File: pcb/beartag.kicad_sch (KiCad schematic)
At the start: 25 parts, among them J1 USB_C_Receptacle_USB2.0_14P, Q1 AO3401A, SW1 SW_Push, SW2 SW_Push, U1 CH571F, U2 XC6206P332MR, Y1 32 MHz, Y2 32.768 kHz

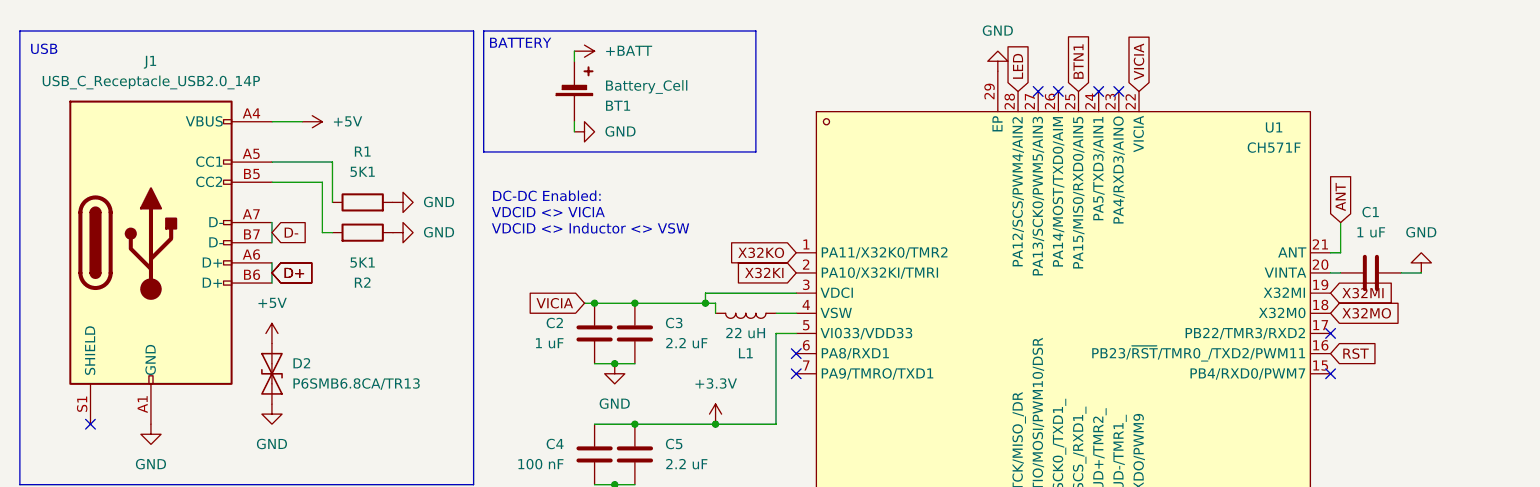
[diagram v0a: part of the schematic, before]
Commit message: pcb updates
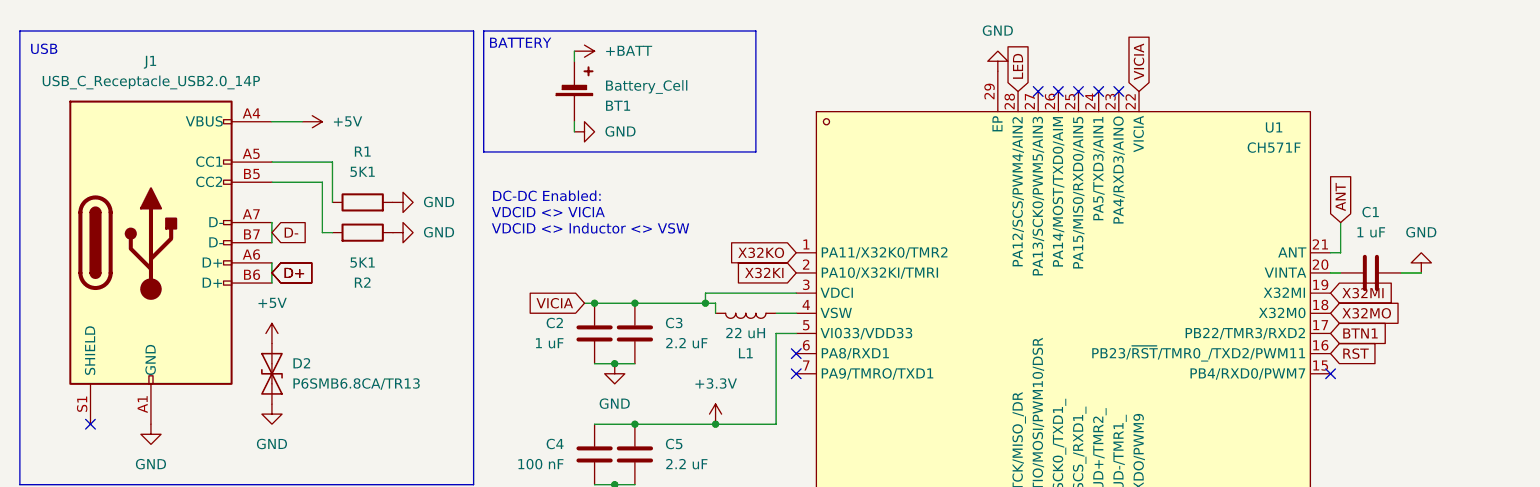
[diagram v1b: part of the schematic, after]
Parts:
- D3: LCSC (none) -> C2286
- R3: LCSC C2286 -> C25905
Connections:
- net BTN1: now also U1.17 (PB22/TMR3/RXD2); no longer U1.25 (PA15/MIS0/RXD0/AIN5)
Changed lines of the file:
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@@
 (kicad_sch
-	(version 20231120)
+	(version 20250114)
 	(generator "eeschema")
-	(generator_version "8.0")
+	(generator_version "9.0")
 	(paper "A4")
+	(rectangle
+		(start 219.71 13.97)
+		(end 252.73 33.02)
+		(stroke
+			(width 0)
+			(type default)
+		)
+		(fill
+			(type none)
+		)
+	)
+	(rectangle
+		(start 100.33 95.25)
+		(end 144.78 128.27)
+		(stroke
+			(width 0)
+			(type default)
+		)
+		(fill
+			(type none)
+		)
+	)
+	(rectangle
+		(start 71.12 12.7)
+		(end 105.41 27.94)
+		(stroke
+			(width 0)
+			(type default)
+		)
+		(fill
+			(type none)
+		)
+	)
+	(rectangle
+		(start 254 13.97)
+		(end 283.21 44.45)
+		(stroke
+			(width 0)
+			(type default)
+		)
+		(fill
+			(type none)
+		)
+	)
+	(rectangle
+		(start 12.7 12.7)
+		(end 69.85 69.85)
+		(stroke
+			(width 0)
+			(type default)
+		)
+		(fill
+			(type none)
+		)
+	)
+	(rectangle
+		(start 12.7 71.12)
+		(end 62.23 95.25)
+		(stroke
+			(width 0)
+			(type default)
+		)
+		(fill
+			(type none)
+		)
+	)
+	(rectangle
+		(start 12.7 97.79)
+		(end 59.69 121.92)
+		(stroke
+			(width 0)
+			(type default)
+		)
+		(fill
+			(type none)
+		)
+	)
+	(rectangle
+		(start 60.96 97.79)
+		(end 93.98 113.03)
+		(stroke
+			(width 0)
+			(type default)
+		)
+		(fill
+			(type none)
+		)
+	)
+	(text "DC-DC Enabled:\nVDCID <> VICIA\nVDCID <> Inductor <> VSW"
+		(exclude_from_sim no)
+		(at 72.136 35.814 0)
+		(effects
+			(font
+				(size 1.27 1.27)
+				(color 0 194 194 1)
+			)
+			(justify left)
+		)
+	)
+	(text "CONTROL BUTTONS"
+		(exclude_from_sim no)
+		(at 22.352 100.33 0)
+		(effects
+			(font
+				(size 1.27 1.27)
+			)
+		)
+	)
+	(text "USB"
+		(exclude_from_sim no)
+		(at 15.748 15.24 0)
+		(effects
+			(font
+				(size 1.27 1.27)
+			)
+		)
+	)
+	(text "LDO"
+		(exclude_from_sim no)
+		(at 15.494 74.168 0)
+		(effects
+			(font
+				(size 1.27 1.27)
+			)
+		)
+	)
+	(text "LOAD SHARING"
+		(exclude_from_sim no)
+		(at 108.458 97.79 0)
+		(effects
+			(font
+				(size 1.27 1.27)
+			)
+		)
+	)
+	(text "ANTENNA"
+		(exclude_from_sim no)
+		(at 225.044 16.002 0)
+		(effects
+			(font
+				(size 1.27 1.27)
+			)
+		)
+	)
+	(text "LED"
+		(exclude_from_sim no)
+		(at 63.5 100.076 0)
+		(effects
+			(font
+				(size 1.27 1.27)
+			)
+		)
+	)
+	(text "BATTERY"
+		(exclude_from_sim no)
+		(at 75.692 14.478 0)
+		(effects
+			(font
+				(size 1.27 1.27)
+			)
+		)
+	)
+	(text "CRYSTALS"
+		(exclude_from_sim no)
+		(at 258.826 16.002 0)
+		(effects
+			(font
+				(size 1.27 1.27)
+			)
+		)
+	)
 	(junction
 		(at 130.81 116.84)
@@
 	)
 	(no_connect
+		(at 146.05 20.32)
+	)
+	(no_connect
 		(at 140.97 20.32)
 	)
@@
 	)
 	(no_connect
-		(at 177.8 50.8)
-	)
-	(no_connect
 		(at 140.97 78.74)
 	)
@@
 		)
 	)
-	(rectangle
-		(start 219.71 13.97)
-		(end 252.73 33.02)
-		(stroke
-			(width 0)
-			(type default)
-		)
-		(fill
-			(type none)
-		)
-	)
-	(rectangle
-		(start 100.33 95.25)
-		(end 144.78 128.27)
-		(stroke
-			(width 0)
-			(type default)
-		)
-		(fill
-			(type none)
-		)
-	)
-	(rectangle
-		(start 71.12 12.7)
-		(end 105.41 27.94)
-		(stroke
-			(width 0)
-			(type default)
-		)
-		(fill
-			(type none)
-		)
-	)
-	(rectangle
-		(start 254 13.97)
-		(end 283.21 44.45)
-		(stroke
-			(width 0)
-			(type default)
-		)
-		(fill
-			(type none)
-		)
-	)
-	(rectangle
-		(start 12.7 12.7)
-		(end 69.85 69.85)
-		(stroke
-			(width 0)
-			(type default)
-		)
-		(fill
-			(type none)
-		)
-	)
-	(rectangle
-		(start 12.7 71.12)
-		(end 62.23 95.25)
-		(stroke
-			(width 0)
-			(type default)
-		)
-		(fill
-			(type none)
-		)
-	)
-	(rectangle
-		(start 12.7 97.79)
-		(end 59.69 121.92)
-		(stroke
-			(width 0)
-			(type default)
-		)
-		(fill
-			(type none)
-		)
-	)
-	(rectangle
-		(start 60.96 97.79)
-		(end 93.98 113.03)
-		(stroke
-			(width 0)
-			(type default)
-		)
-		(fill
-			(type none)
-		)
-	)
-	(text "DC-DC Enabled:\nVDCID <> VICIA\nVDCID <> Inductor <> VSW"
-		(exclude_from_sim no)
-		(at 72.136 35.814 0)
-		(effects
-			(font
-				(size 1.27 1.27)
-				(color 0 194 194 1)
-			)
-			(justify left)
-		)
-	)
-	(text "CONTROL BUTTONS"
-		(exclude_from_sim no)
-		(at 22.352 100.33 0)
-		(effects
-			(font
-				(size 1.27 1.27)
-			)
-		)
-	)
-	(text "USB"
-		(exclude_from_sim no)
-		(at 15.748 15.24 0)
-		(effects
-			(font
-				(size 1.27 1.27)
-			)
-		)
-	)
-	(text "LDO"
-		(exclude_from_sim no)
-		(at 15.494 74.168 0)
-		(effects
-			(font
-				(size 1.27 1.27)
-			)
-		)
-	)
-	(text "LOAD SHARING"
-		(exclude_from_sim no)
-		(at 108.458 97.79 0)
-		(effects
-			(font
-				(size 1.27 1.27)
-			)
-		)
-	)
-	(text "ANTENNA"
-		(exclude_from_sim no)
-		(at 225.044 16.002 0)
-		(effects
-			(font
-				(size 1.27 1.27)
-			)
-		)
-	)
-	(text "LED"
-		(exclude_from_sim no)
-		(at 63.5 100.076 0)
-		(effects
-			(font
-				(size 1.27 1.27)
-			)
-		)
-	)
-	(text "BATTERY"
-		(exclude_from_sim no)
-		(at 75.692 14.478 0)
-		(effects
-			(font
-				(size 1.27 1.27)
-			)
-		)
-	)
-	(text "CRYSTALS"
-		(exclude_from_sim no)
-		(at 258.826 16.002 0)
-		(effects
-			(font
-				(size 1.27 1.27)
-			)
-		)
-	)
 	(global_label "X32KI"
 		(shape input)
@@
 		)
 	)
-	(global_label "BTN1"
-		(shape input)
-		(at 146.05 20.32 90)
-		(fields_autoplaced yes)
-		(effects
-			(font
-				(size 1.27 1.27)
-			)
-			(justify left)
-		)
-		(property "Intersheetrefs" "${INTERSHEET_REFS}"
-			(at 146.05 12.5572 90)
-			(effects
-				(font
-					(size 1.27 1.27)
-				)
-				(justify left)
-				(hide yes)
-			)
-		)
-	)
 	(global_label "RST"
 		(shape input)
@@
 		)
 	)
+	(global_label "BTN1"
+		(shape input)
+		(at 177.8 50.8 0)
+		(fields_autoplaced yes)
+		(effects
+			(font
+				(size 1.27 1.27)
+			)
+			(justify left)
+		)
+		(property "Intersheetrefs" "${INTERSHEET_REFS}"
+			(at 185.5628 50.8 0)
+			(effects
+				(font
+					(size 1.27 1.27)
+				)
+				(justify left)
+				(hide yes)
+			)
+		)
+	)
 	(global_label "X32MO"
 		(shape input)
@@
 			)
 		)
+		(property "LCSC" "C2286"
+			(at 74.93 107.95 0)
+			(effects
+				(font
+					(size 1.27 1.27)
+				)
+				(hide yes)
+			)
+		)
 		(pin "2"
 		)
@@
 			)
 		)
-		(property "LCSC" "C2286"
+		(property "LCSC" "C25905"
 			(at 82.55 107.95 90)
 			(effects
@@
 		)
 	)
+	(embedded_fonts no)
 )
